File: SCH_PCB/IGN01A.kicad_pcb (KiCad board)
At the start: 2 copper layers, 55 x 45 mm, 21 parts, among them IC1 ATMEGA328-A, J1 PWR, J2 IGN, J3 HEADER_1x11, J5 ISP, Q1 IRF7413ZPBF, U1 MPL3115A2

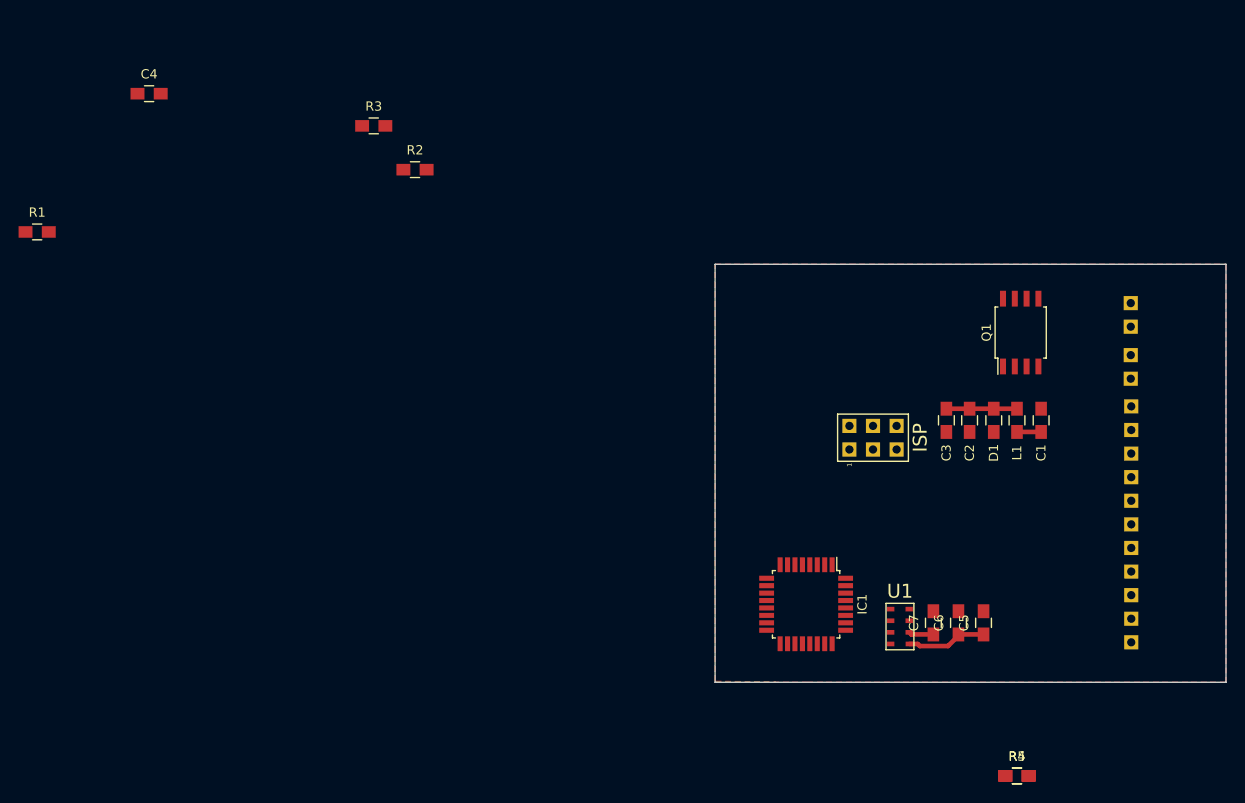
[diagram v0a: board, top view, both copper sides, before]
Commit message: pcb added
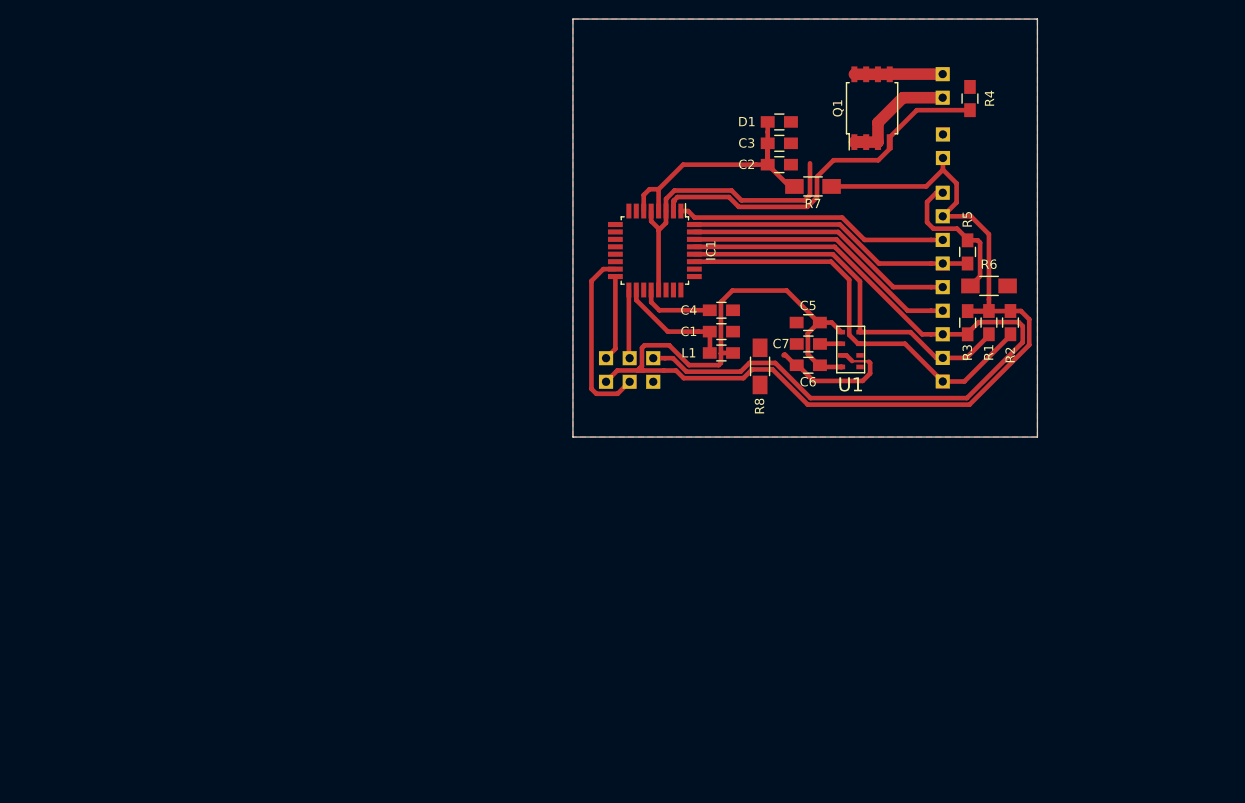
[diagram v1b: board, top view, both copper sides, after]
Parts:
- added R6: 0, Capacitors_SMD:C_1206_HandSoldering, F.Cu at (210.8, 119.7)
- added R7: 0, Capacitors_SMD:C_1206_HandSoldering, F.Cu at (191.8, 109.0)
- added R8: 0, Capacitors_SMD:C_1206_HandSoldering, F.Cu at (186.1, 128.4)
- J3: value HEADER_1x11 -> HEADER_1x09; footprint Mlab_Pin_Headers:Angled_1x11 -> Mlab_Pin_Headers:Angled_1x09
- J5: moved to B.Cu
- moved R1 102.9 mm to (210.8, 123.7), turned to 270 degrees
- moved R4 73.1 mm to (208.7, 99.6), turned to 90 degrees
- moved R3 67.4 mm to (208.5, 123.7), turned to 270 degrees
- moved R2 66.2 mm to (213.1, 123.7), turned to 270 degrees
- moved C4 65.9 mm to (182.0, 122.3)
- moved R5 56.7 mm to (208.5, 116.1), turned to 90 degrees
- moved IC1 41.4 mm to (174.8, 115.9)
- moved D1 39.6 mm to (188.2, 102.1), turned to 0 degrees
- moved C5 37.4 mm to (191.3, 123.7), turned to 180 degrees
- moved C1 35.7 mm to (182.0, 124.7), turned to 0 degrees
- moved C3 34.8 mm to (188.2, 104.4), turned to 0 degrees
- moved C2 34.3 mm to (188.2, 106.7), turned to 0 degrees
- moved C7 32.9 mm to (191.3, 126.0), turned to 180 degrees
- moved L1 32.6 mm to (182.0, 127.0), turned to 0 degrees
- moved J3 32.6 mm to (205.8, 119.9)
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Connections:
- IC1 pad 1: /PD3 -> /OUT
- IC1 pad 2: /PD4 -> /IGN
- IC1 pad 32: /PD2 -> /IN
- J3 pad 3: /PD3 -> /RST
- J3 pad 4: GND -> /RXD
- J3 pad 5: /RXD -> /TXD
- J3 pad 6: /TXD -> /IN
- J3 pad 7: GND -> /OUT
- J3 pad 9: /RST -> GND
- Q1 pad 4: /PD2 -> /IGN
- R4 pad 1: /PD2 -> /IGN
- R5 pad 1: /PD3 -> /IN
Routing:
- net VDD: track 16.3 -> 171.4 mm
- net /RST: track 0.00 -> 86.6 mm
- net GND: track 0.00 -> 64.0 mm
- net /SDA: track 0.00 -> 45.2 mm
- net /SCL: track 0.00 -> 40.7 mm
- net /IGN: track 0.00 -> 40.1 mm
- net /IN: track 0.00 -> 31.2 mm
- net /RXD: track 0.00 -> 29.9 mm
- net /OUT: track 0.00 -> 29.9 mm
- net /TXD: track 0.00 -> 29.2 mm
- net /MOSI: track 0.00 -> 19.6 mm
- net Net-(J2-Pad1): track 0.00 -> 14.0 mm
- net VAA: track 2.60 -> 12.8 mm
- net Net-(J2-Pad2): track 0.00 -> 9.51 mm
- net /MISO: track 0.00 -> 9.21 mm
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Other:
- board size 55 x 45 mm -> 50 x 45 mm
- net class Default: trace_width 0.5 -> 0.25
- net class PWR removed
- rule pad_to_mask_clearance: 0.2 -> 0
- board text added: "IN"
- board text added: "OUT"
- board text removed: "A"
- board text removed: "C"
- board text removed: "GND"
- board text removed: "PD3"
- board text removed: "PD4"
- board text removed: "VDD"
